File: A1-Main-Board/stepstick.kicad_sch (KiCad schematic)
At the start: 18 parts, among them J1 Conn_01x04, U1 TMC2209-LA

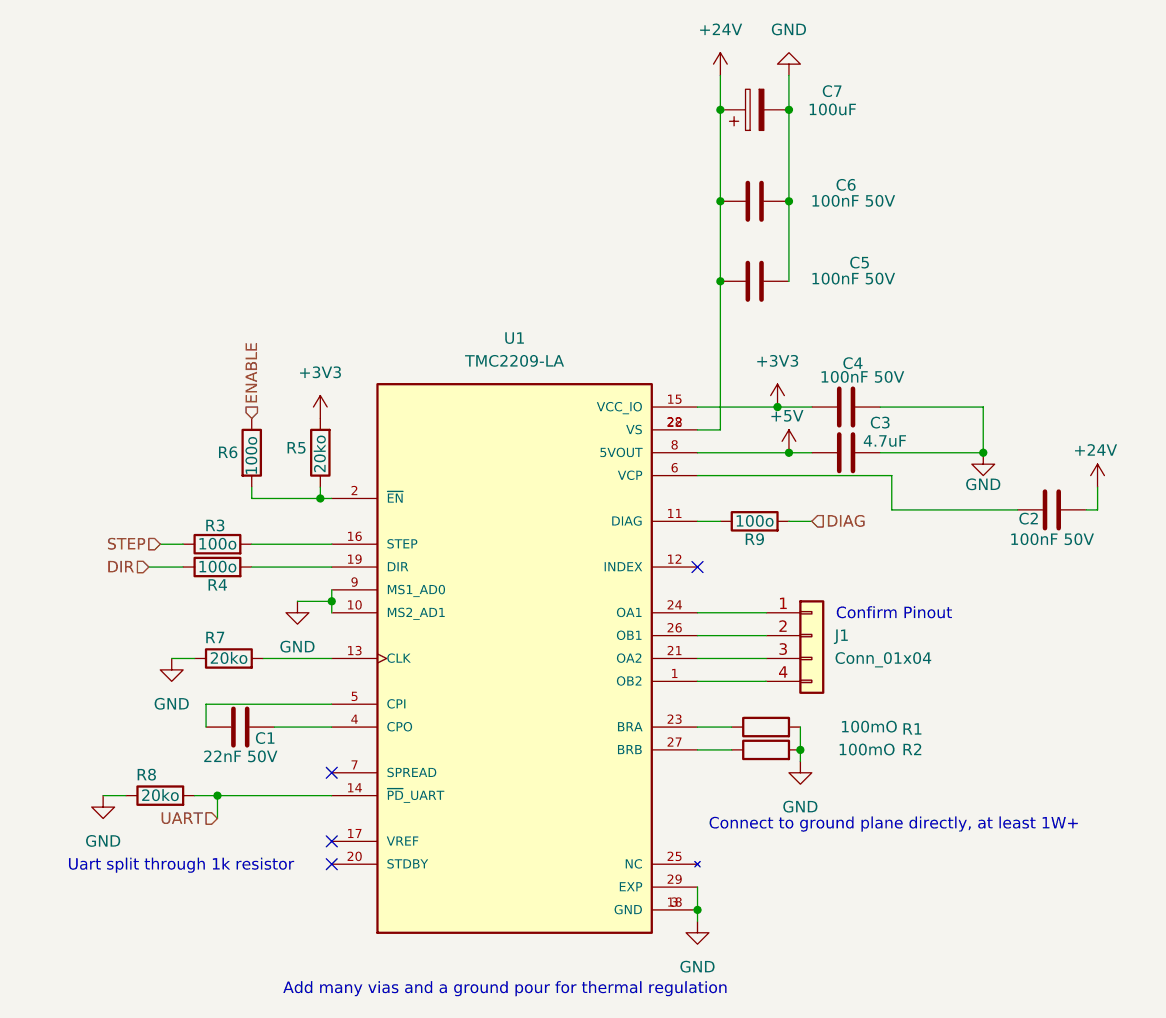
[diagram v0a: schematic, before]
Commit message: e
e
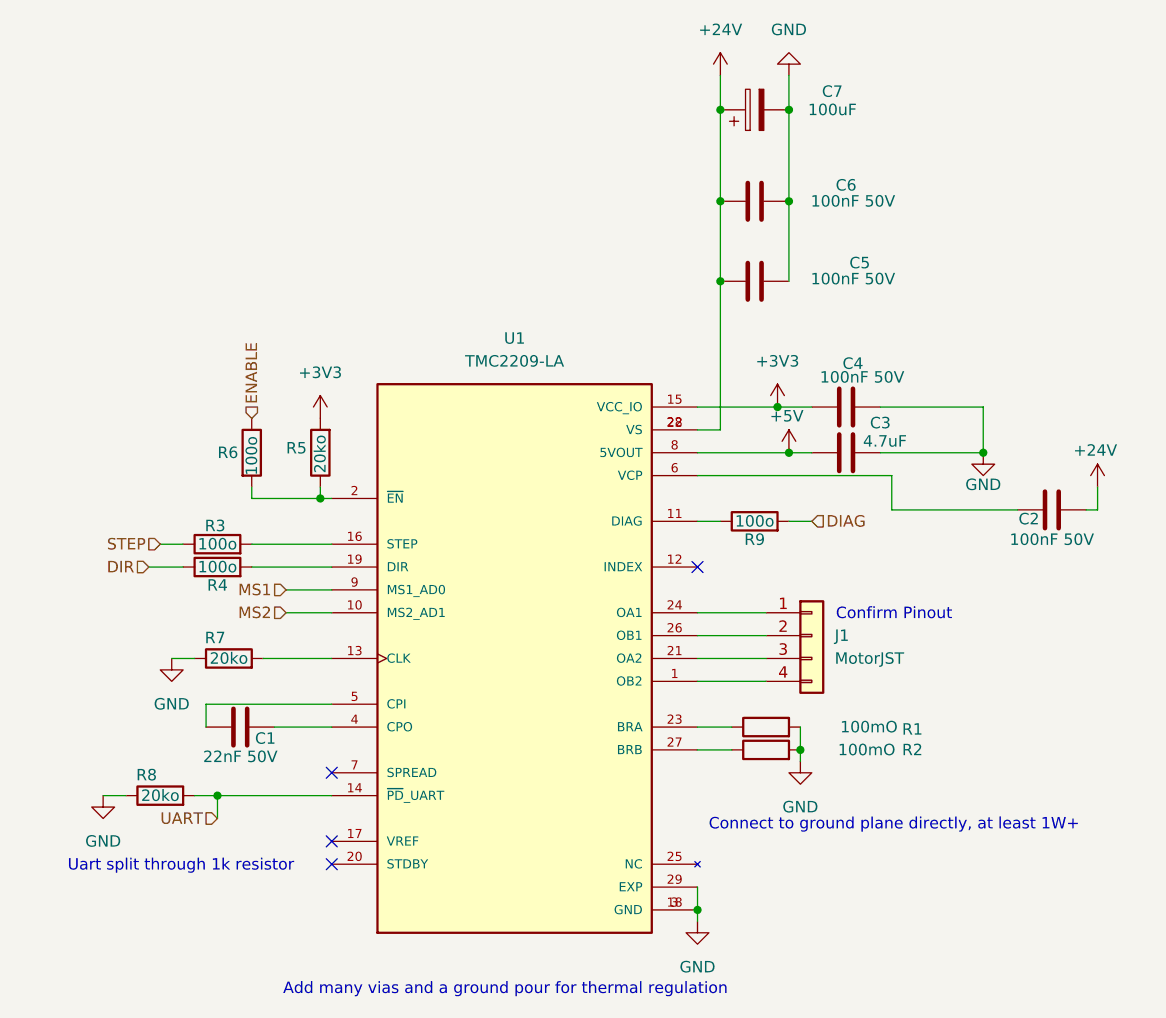
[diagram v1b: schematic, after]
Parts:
- J1: value Conn_01x04 -> MotorJST; footprint (none) -> Connector_JST:JST_XH_B4B-XH-A_1x04_P2.50mm_Vertical
- U1: footprint TMC2209-LA:QFN50P500X500X90-29N -> footprints:TMC2209-LA
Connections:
- net GND: no longer U1.10 (MS2_AD1), U1.9 (MS1_AD0)
- new net MS1: U1.9 (MS1_AD0)
- new net MS2: U1.10 (MS2_AD1)
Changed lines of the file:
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@@
-	)
-	(junction
-		(at 44.45 83.82)
-		(diameter 0)
-		(color 0 0 0 0)
 	)
 	(junction
@@
 	(wire
 		(pts
-			(xy 40.64 83.82) (xy 44.45 83.82)
-		)
-		(stroke
-			(width 0)
-			(type default)
-		)
-	)
-	(wire
-		(pts
 			(xy 25.4 77.47) (xy 27.94 77.47)
 		)
@@
 	(wire
 		(pts
-			(xy 44.45 82.55) (xy 44.45 83.82)
-		)
-		(stroke
-			(width 0)
-			(type default)
-		)
-	)
-	(wire
-		(pts
-			(xy 44.45 83.82) (xy 44.45 85.09)
-		)
-		(stroke
-			(width 0)
-			(type default)
-		)
-	)
-	(wire
-		(pts
 			(xy 96.52 97.79) (xy 96.52 100.33)
 		)
@@
 	(wire
 		(pts
+			(xy 39.37 85.09) (xy 44.45 85.09)
+		)
+		(stroke
+			(width 0)
+			(type default)
+		)
+	)
+	(wire
+		(pts
 			(xy 97.79 74.93) (xy 95.25 74.93)
 		)
@@
 	(wire
 		(pts
+			(xy 39.37 82.55) (xy 44.45 82.55)
+		)
+		(stroke
+			(width 0)
+			(type default)
+		)
+	)
+	(wire
+		(pts
 			(xy 129.54 73.66) (xy 128.27 73.66)
 		)
@@
 			(width 0)
 			(type default)
+		)
+	)
+	(hierarchical_label "MS2"
+		(shape input)
+		(at 39.37 85.09 180)
+		(effects
+			(font
+				(size 1.27 1.27)
+			)
+			(justify right)
 		)
 	)
@@
 		(shape input)
 		(at 24.13 80.01 180)
+		(effects
+			(font
+				(size 1.27 1.27)
+			)
+			(justify right)
+		)
+	)
+	(hierarchical_label "MS1"
+		(shape input)
+		(at 39.37 82.55 180)
 		(effects
 			(font
@@
 			)
 		)
-		(property "Footprint" "TMC2209-LA:QFN50P500X500X90-29N"
+		(property "Footprint" "footprints:TMC2209-LA"
 			(at 64.77 90.17 0)
 			(effects
@@
 	)
 	(symbol
-		(lib_id "power:GND")
-		(at 40.64 83.82 0)
-		(unit 1)
-		(exclude_from_sim no)
-		(in_bom yes)
-		(on_board yes)
-		(dnp no)
-		(fields_autoplaced yes)
-		(property "Reference" "#PWR03"
-			(at 40.64 90.17 0)
-			(effects
-				(font
-					(size 1.27 1.27)
-				)
-				(hide yes)
-			)
-		)
-		(property "Value" "GND"
-			(at 40.64 88.9 0)
-			(effects
-				(font
-					(size 1.27 1.27)
-				)
-			)
-		)
-		(property "Footprint" ""
-			(at 40.64 83.82 0)
-			(effects
-				(font
-					(size 1.27 1.27)
-				)
-				(hide yes)
-			)
-		)
-		(property "Datasheet" ""
-			(at 40.64 83.82 0)
-			(effects
-				(font
-					(size 1.27 1.27)
-				)
-				(hide yes)
-			)
-		)
-		(property "Description" "Power symbol creates a global label with name \"GND\" , ground"
-			(at 40.64 83.82 0)
-			(effects
-				(font
-					(size 1.27 1.27)
-				)
-				(hide yes)
-			)
-		)
-		(pin "1"
-		)
-		(instances
-			(project "A1-Main-Board"
-				(path "/9d813fc3-a6a1-4e23-ab17-d125b692e1a2/c4b8059d-0776-437d-bd29-86172f3939cd/870b9616-0713-440f-86ea-848a0e7cfb1d"
-					(reference "#PWR030")
-					(unit 1)
-				)
-				(path "/9d813fc3-a6a1-4e23-ab17-d125b692e1a2/c4b8059d-0776-437d-bd29-86172f3939cd/9f561cc0-cecc-4b9d-8c7a-f3aaac7544b7"
-					(reference "#PWR015")
-					(unit 1)
-				)
-				(path "/9d813fc3-a6a1-4e23-ab17-d125b692e1a2/c4b8059d-0776-437d-bd29-86172f3939cd/c3aa2540-bff6-4275-a49d-0ccfa2e7a55c"
-					(reference "#PWR03")
-					(unit 1)
-				)
-			)
-		)
-	)
-	(symbol
 		(lib_id "Connector_Generic:Conn_01x04")
 		(at 97.79 87.63 0)
@@
 			)
 		)
-		(property "Value" "Conn_01x04"
+		(property "Value" "MotorJST"
 			(at 100.33 90.1699 0)
 			(effects
@@
 			)
 		)
-		(property "Footprint" ""
+		(property "Footprint" "Connector_JST:JST_XH_B4B-XH-A_1x04_P2.50mm_Vertical"
 			(at 97.79 87.63 0)
 			(effects
